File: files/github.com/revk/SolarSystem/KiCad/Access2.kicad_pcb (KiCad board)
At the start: 2 copper layers, 50 x 26.5 mm, 65 parts, among them J1 USB-C, J2 RFID, J3 INPUTS, J5 POWER, J6 DOOR, Q1 NX7002AK, SW1 ESE13V01D, U1 ESP32-PICO-MINI-02, U2 FT231XQ, U3 G3VM-41GR8, U4 LMR16006+FB, U5 LMR16006+FB, U6 AA, U7 QR

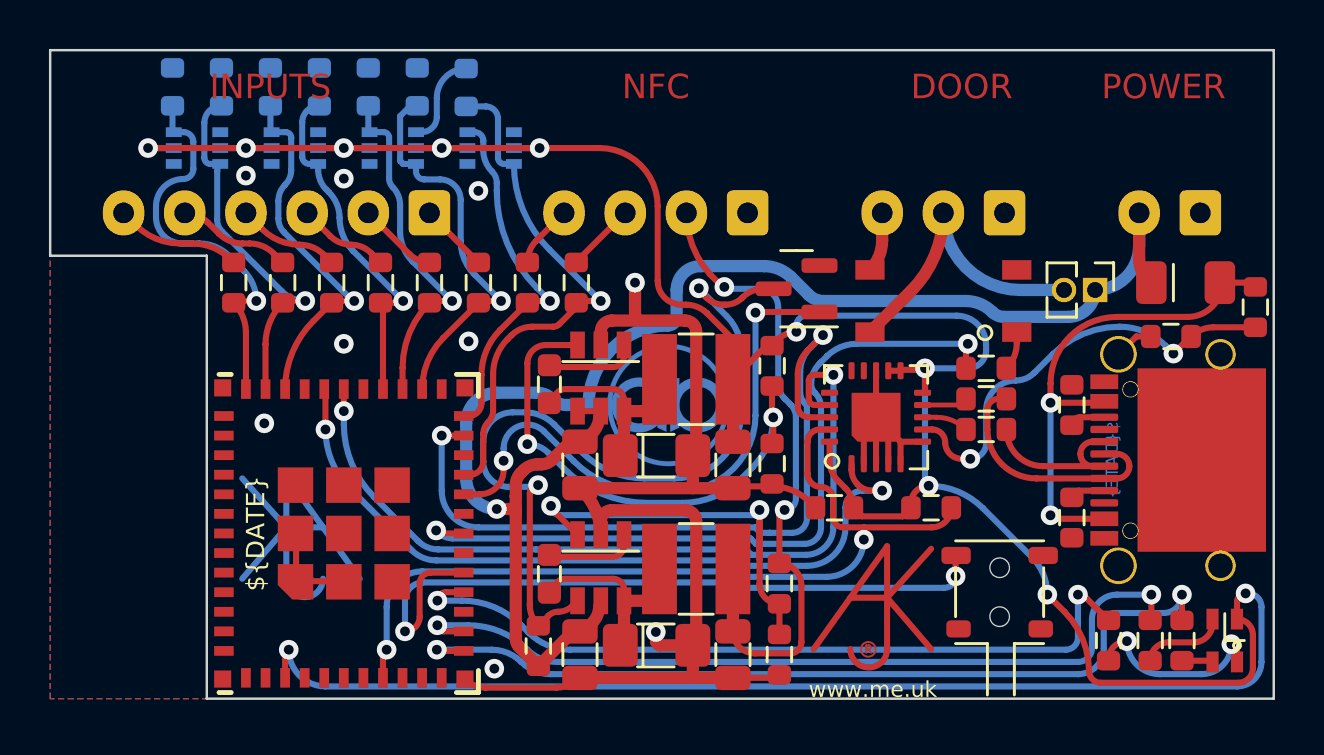
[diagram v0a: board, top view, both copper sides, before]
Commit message: Include .kicad_pro
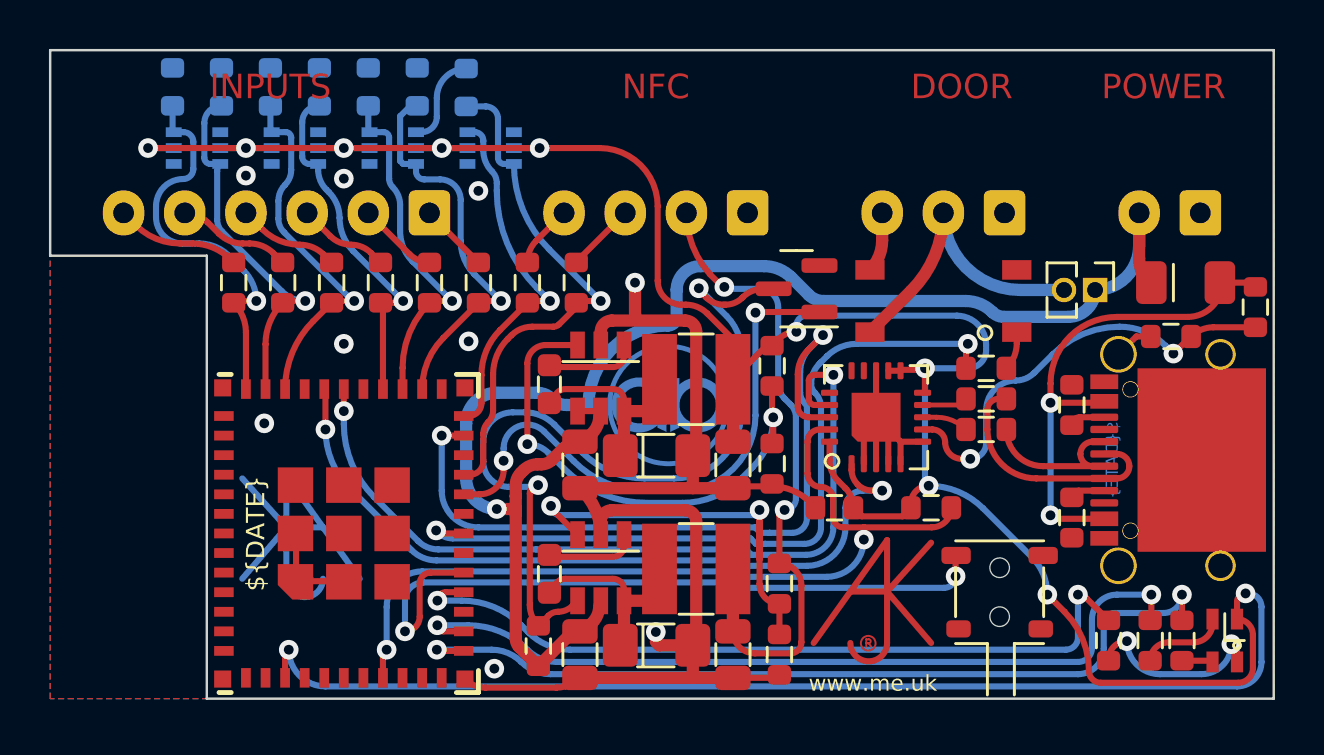
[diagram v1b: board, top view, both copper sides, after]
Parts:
- moved Logo1 0.25 mm to (134.2, 88.1)
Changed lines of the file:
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@@
 (kicad_pcb (version 20211014) (generator pcbnew)
   (general
-    (thickness 1.6)
+    (thickness 0.8)
   )
   (paper "A4")
@@
       (layer "F.SilkS" (type "Top Silk Screen"))
       (layer "F.Paste" (type "Top Solder Paste"))
-      (layer "F.Mask" (type "Top Solder Mask") (thickness 0.01))
+      (layer "F.Mask" (type "Top Solder Mask") (color "Purple") (thickness 0.01))
       (layer "F.Cu" (type "copper") (thickness 0.035))
-      (layer "dielectric 1" (type "core") (thickness 1.51) (material "FR4") (epsilon_r 4.5) (loss_tangent 0.02))
+      (layer "dielectric 1" (type "core") (thickness 0.71) (material "FR4") (epsilon_r 4.5) (loss_tangent 0.02))
       (layer "B.Cu" (type "copper") (thickness 0.035))
-      (layer "B.Mask" (type "Bottom Solder Mask") (thickness 0.01))
+      (layer "B.Mask" (type "Bottom Solder Mask") (color "Purple") (thickness 0.01))
       (layer "B.Paste" (type "Bottom Solder Paste"))
       (layer "B.SilkS" (type "Bottom Silk Screen"))
@@
     (fp_line (start 3.7 6.6) (end -3.7 6.6) (layer "F.Fab") (width 0.12))
     (fp_line (start -2.7 -1.3) (end -3.7 -0.3) (layer "F.Fab") (width 0.12))
-    (pad "1" thru_hole roundrect (at -1.25 0 180) (size 1.7 1.85) (drill 0.85) (layers *.Cu *.Mask) (roundrect_rratio 0.147059)
+    (pad "1" thru_hole roundrect (at -1.25 0 180) (size 1.7 1.85) (drill 0.85) (layers *.Cu *.Mask) (roundrect_rratio 0.1470588235)
       (net 3 "GND") (pinfunction "GND") (pintype "power_in"))
     (pad "2" thru_hole oval (at 1.25 0 180) (size 1.7 1.85) (drill 0.85) (layers *.Cu *.Mask)
@@
     (fp_line (start 0 2) (end -1 3) (layer "F.Fab") (width 0.12))
     (fp_line (start 0 5) (end 0 2) (layer "F.Fab") (width 0.12))
-    (pad "1" thru_hole roundrect (at -2.5 0 180) (size 1.7 1.85) (drill 0.85) (layers *.Cu *.Mask) (roundrect_rratio 0.147059)
+    (pad "1" thru_hole roundrect (at -2.5 0 180) (size 1.7 1.85) (drill 0.85) (layers *.Cu *.Mask) (roundrect_rratio 0.1470588235)
       (net 3 "GND") (pinfunction "Pin_1") (pintype "passive"))
     (pad "2" thru_hole oval (at 0 0 180) (size 1.7 1.85) (drill 0.85) (layers *.Cu *.Mask)
@@
     (fp_line (start -6.2 6.6) (end -6.2 -1.3) (layer "F.Fab") (width 0.12))
     (fp_line (start 6.2 -1.3) (end 6.2 6.6) (layer "F.Fab") (width 0.12))
-    (pad "1" thru_hole roundrect (at -3.75 0 180) (size 1.7 1.85) (drill 0.85) (layers *.Cu *.Mask) (roundrect_rratio 0.147059)
+    (pad "1" thru_hole roundrect (at -3.75 0 180) (size 1.7 1.85) (drill 0.85) (layers *.Cu *.Mask) (roundrect_rratio 0.1470588235)
       (net 3 "GND") (pinfunction "Pin_1") (pintype "passive"))
     (pad "2" thru_hole oval (at -1.25 0 180) (size 1.7 1.85) (drill 0.85) (layers *.Cu *.Mask)
@@
     (fp_line (start 0 5) (end 0 2) (layer "F.Fab") (width 0.12))
     (fp_line (start 0 2) (end 1 3) (layer "F.Fab") (width 0.12))
-    (pad "1" thru_hole roundrect (at -6.25 0 180) (size 1.7 1.85) (drill 0.85) (layers *.Cu *.Mask) (roundrect_rratio 0.147059)
+    (pad "1" thru_hole roundrect (at -6.25 0 180) (size 1.7 1.85) (drill 0.85) (layers *.Cu *.Mask) (roundrect_rratio 0.1470588235)
       (net 37 "Net-(J3-Pad1)") (pinfunction "Pin_1") (pintype "passive"))
     (pad "2" thru_hole oval (at -3.75 0 180) (size 1.7 1.85) (drill 0.85) (layers *.Cu *.Mask)
@@
   )
   (footprint "RevK:AJK" (layer "F.Cu")
-    (at 134.2 88.375)
+    (at 134.2 88.125)
     (property "Note" "Non part, PCB printed")
     (property "Sheetfile" "Access2.kicad_sch")
